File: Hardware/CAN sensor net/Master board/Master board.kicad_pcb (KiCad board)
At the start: 2 copper layers, 72 parts, among them J1 Micro_SD_Card_Con, J2 USB_B_Micro, J3 Conn_02x05_SWD, J4 XT60, J5 532610671, J6 532610671, J7 DC-005, SW1 SW_Push, SW2 SW_SPDT, U1 STM32F405RGTx, U2 USBLC6-2SC6, U3 ST1S14PHR, U4 LDL1117_3V3, U5 SN65HVD230, U6 SN65HVD230, Y1 16MHz

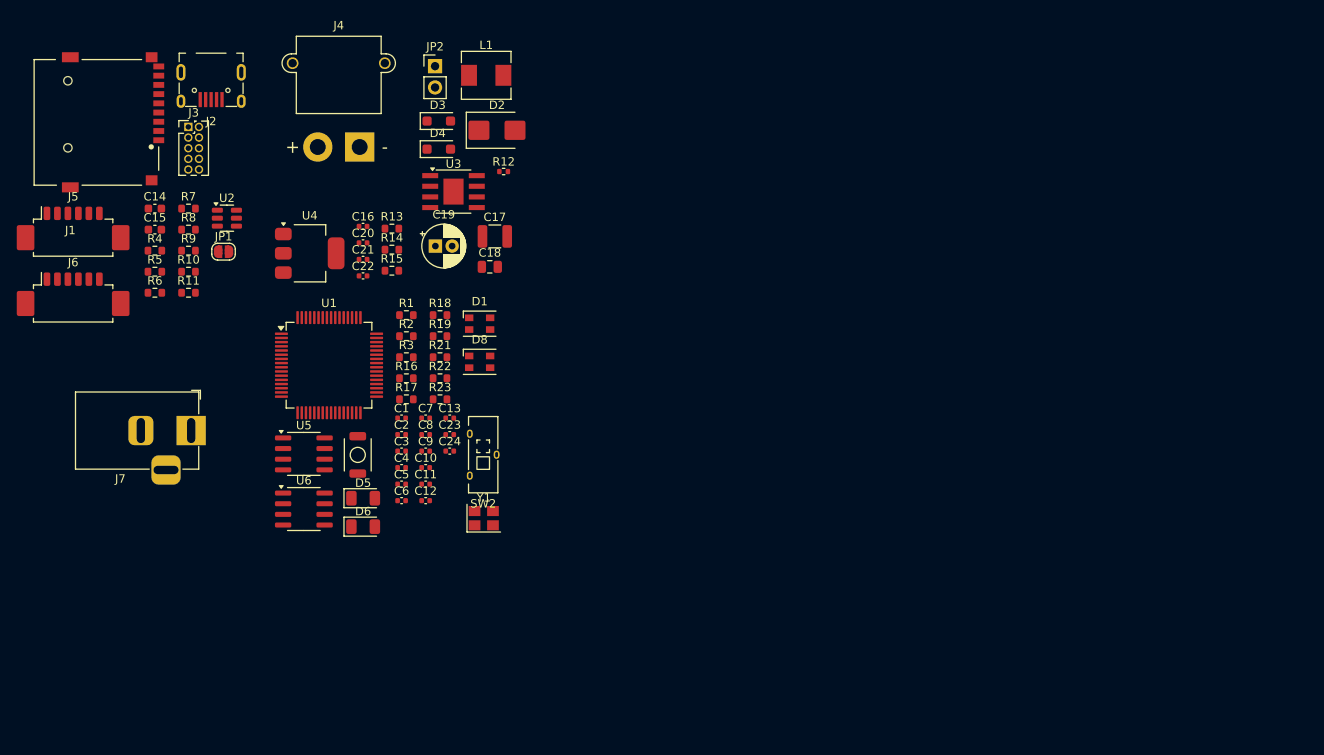
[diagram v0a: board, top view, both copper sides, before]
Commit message: Master board сoncept
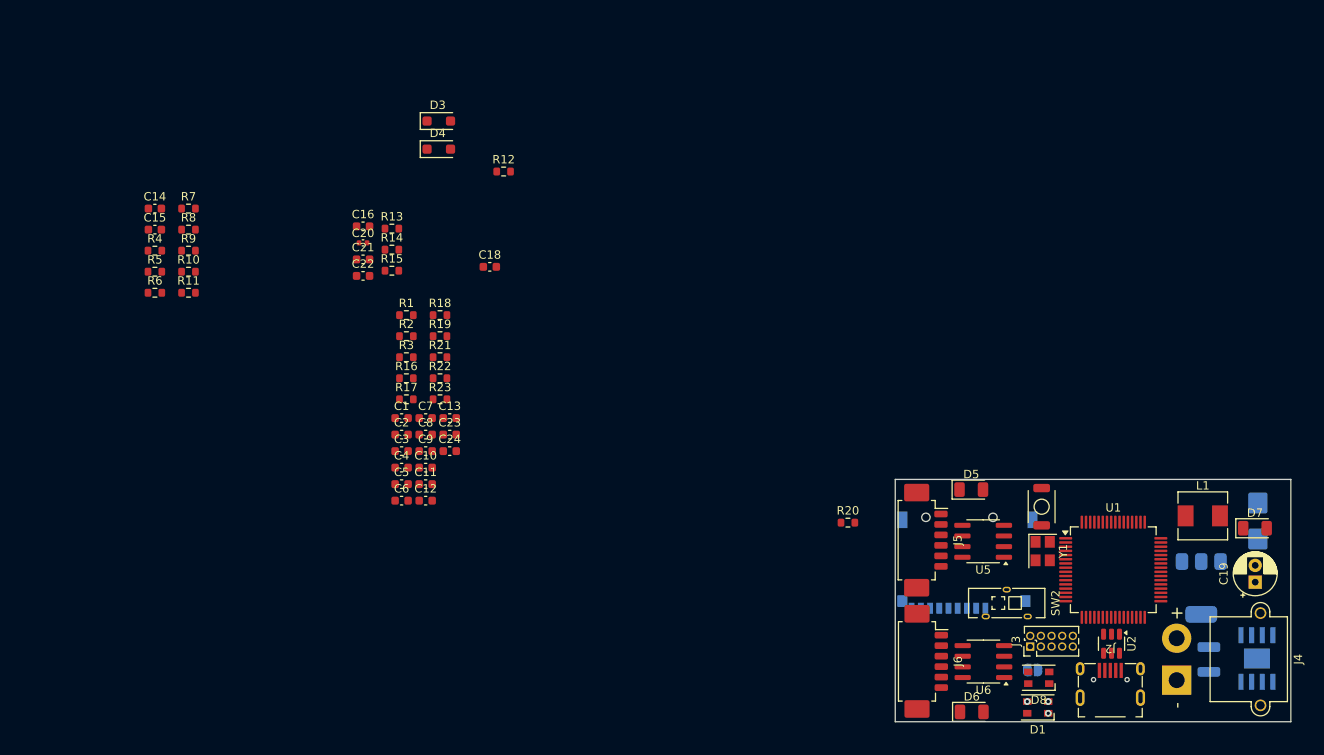
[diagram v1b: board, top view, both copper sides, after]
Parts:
- removed J7: DC-005, Connector_BarrelJack:BarrelJack_Horizontal
- removed JP2: Jumper_2_Bridged, Connector_PinHeader_2.54mm:PinHeader_1x02_P2.54mm_Vertical
- added D7: LED, LED_SMD:LED_1206_3216Metric, F.Cu at (213.1, 90.0)
- added R20: 220, Resistor_SMD:R_0603_1608Metric, F.Cu at (164.5, 89.3)
- C1, C10, C11, C12, C13, C16, C2, C21, C22, C23, C24, C3, C4, C5, C6, C7, C8, C9: footprint Capacitor_SMD:C_0402_1005Metric -> Capacitor_SMD:C_0603_1608Metric
- C17, D2, J1, JP1, U3, U4: moved to B.Cu
- C18: footprint Capacitor_SMD:C_0805_2012Metric -> Capacitor_SMD:C_0603_1608Metric
- R12: footprint Resistor_SMD:R_0402_1005Metric -> Resistor_SMD:R_0603_1608Metric
- moved J2 130.6 mm to (195.8, 110.2), turned to 180 degrees
- moved J1 121.4 mm to (186.6, 88.9), turned to -90 degrees
- moved J3 118.0 mm to (186.3, 104.1), turned to 90 degrees
- moved U2 117.1 mm to (196.0, 103.7), turned to -90 degrees
- moved J4 116.4 mm to (203.8, 108.1), turned to -90 degrees
- moved U4 113.6 mm to (206.7, 97.1), turned to -90 degrees
- moved U3 110.8 mm to (213.3, 105.5), turned to -90 degrees
- moved J6 110.0 mm to (173.3, 105.8), turned to -90 degrees
- moved JP1 108.6 mm to (186.6, 106.9), turned to 180 degrees
- moved J5 107.5 mm to (173.2, 91.4), turned to -90 degrees
- moved C19 105.7 mm to (213.1, 96.4), turned to 90 degrees
- moved D2 102.0 mm to (213.4, 89.1), turned to -90 degrees
- moved L1 100.3 mm to (206.9, 88.5)
- moved C17 99.0 mm to (207.6, 105.6), turned to 90 degrees
- moved U1 96.7 mm to (196.2, 94.9)
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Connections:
- C22 pad 1: Net-(JP2-A) -> VDD_3V3
- U4 pad 2: Net-(JP2-A) -> VDD_3V3
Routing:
- net Net-(D1-RK): vias 0 -> 1
- net Net-(D1-GK): vias 0 -> 1
- net Net-(D1-BK): vias 0 -> 1
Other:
- board outline added: 47.2 x 28.9 mm
